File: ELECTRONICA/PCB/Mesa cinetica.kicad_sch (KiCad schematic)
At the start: 0 parts

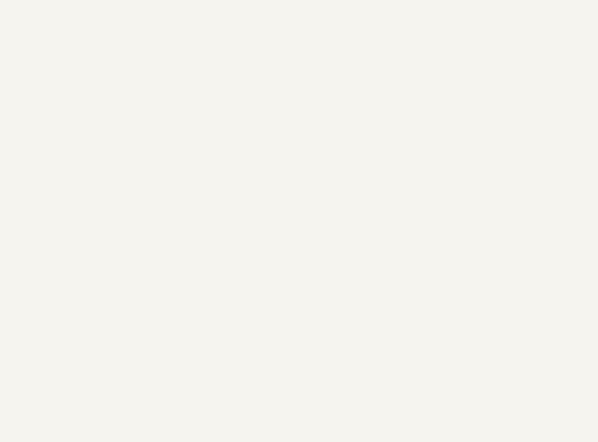
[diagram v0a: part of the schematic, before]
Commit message: Estructura inicial
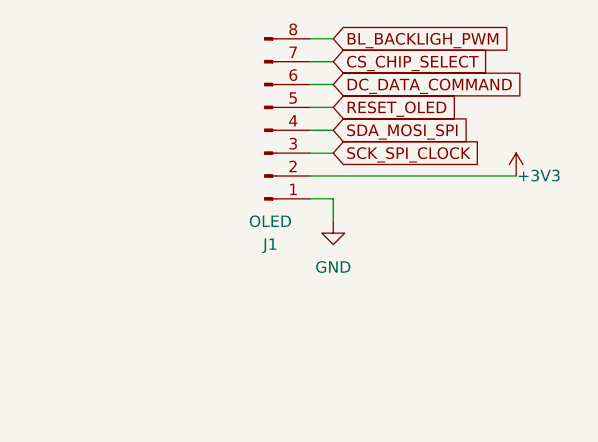
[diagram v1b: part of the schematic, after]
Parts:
- added J1: OLED, symbol Connector:Conn_01x08_Pin
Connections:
- new net +3V3: J1.2 (Pin_2)
- new net BL_BACKLIGH_PWM: J1.8 (Pin_8)
- new net CS_CHIP_SELECT: J1.7 (Pin_7)
- new net DC_DATA_COMMAND: J1.6 (Pin_6)
- new net GND: J1.1 (Pin_1)
- new net RESET_OLED: J1.5 (Pin_5)
- new net SCK_SPI_CLOCK: J1.3 (Pin_3)
- new net SDA_MOSI_SPI: J1.4 (Pin_4)
